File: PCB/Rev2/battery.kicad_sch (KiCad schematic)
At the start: 10 parts, among them U2 ETA6093

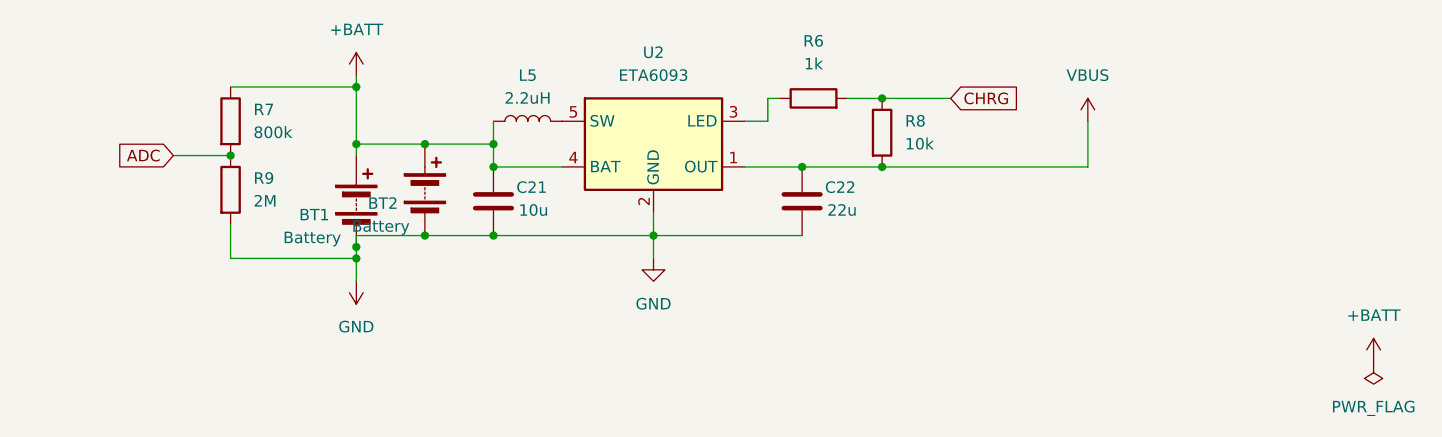
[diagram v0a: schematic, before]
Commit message: drc
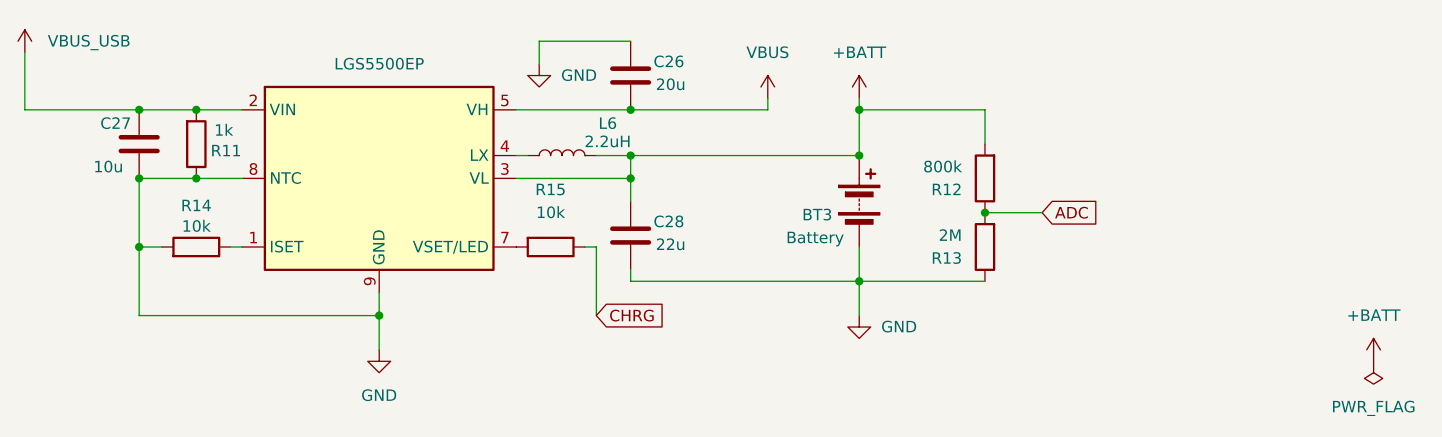
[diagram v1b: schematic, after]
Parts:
- removed BT1, BT2: Battery, Connector_Molex:Molex_PicoBlade_53261-0271_1x02-1MP_P1.25mm_Horizontal, symbol Device:Battery
- removed C21: 10u, Capacitor_SMD:C_0402_1005Metric, symbol Device:C
- removed C22: 22u, Capacitor_SMD:C_0603_1608Metric, symbol Device:C
- removed L5: 2.2uH, Inductor_SMD:L_Changjiang_FNR252012S, symbol Device:L
- removed R6: 1k, PCM_Resistor_SMD_AKL:R_0402_1005Metric, symbol Device:R
- removed R7: 800k, PCM_Resistor_SMD_AKL:R_0603_1608Metric, symbol Device:R
- removed R8: 10k, PCM_Resistor_SMD_AKL:R_0402_1005Metric, symbol Device:R
- removed R9: 2M, PCM_Resistor_SMD_AKL:R_0603_1608Metric, symbol Device:R
- removed U2: ETA6093, Package_TO_SOT_SMD:SOT-23-5, symbol ETA6093:ETA6093
- added BT3: Battery, Connector_Molex:Molex_PicoBlade_53261-0271_1x02-1MP_P1.25mm_Horizontal, symbol Device:Battery
- added C26: 20u, Capacitor_SMD:C_0402_1005Metric, symbol Device:C
- added C27: 10u, Capacitor_SMD:C_0402_1005Metric, symbol Device:C
- added C28: 22u, Capacitor_SMD:C_0603_1608Metric, symbol Device:C
- added L6: 2.2uH, Inductor_SMD:L_Changjiang_FNR252012S, symbol Device:L
- added R11: 1k, PCM_Resistor_SMD_AKL:R_0402_1005Metric, symbol Device:R
- added R12: 800k, PCM_Resistor_SMD_AKL:R_0603_1608Metric, symbol Device:R
- added R13: 2M, PCM_Resistor_SMD_AKL:R_0603_1608Metric, symbol Device:R
- added R14, R15: 10k, PCM_Resistor_SMD_AKL:R_0402_1005Metric, symbol Device:R
- added U4: LGS5500EP, Package_SO:SOIC-8-1EP_3.9x4.9mm_P1.27mm_EP2.41x3.3mm, symbol Battery_Management:LGS5500EP
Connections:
- net +BATT: now also BT3.1 (+), C28.1, L6.2, R12.2, U4.3 (VL)
- net ADC: now also R12.1, R13.2
- net CHRG: now also R15.1
- net GND: now also BT3.2 (-), C26.1, C27.2, C28.2, R11.1, R13.1, R14.2, U4.8 (NTC), U4.9 (GND)
- net VBUS: now also C26.2, U4.5 (VH)
- new net: R15.2, U4.7 (VSET/LED)
- new net: R14.1, U4.1 (ISET)
- new net: L6.1, U4.4 (LX)
- new net VBUS_USB: C27.1, R11.2, U4.2 (VIN)
